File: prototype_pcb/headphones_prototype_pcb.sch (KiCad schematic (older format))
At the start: 51 parts, among them J1 LIGHTING_JACK, J2 CONN_01X10, J3 BOTTOM_FLEX_LIGHTNING, J4 CONN_01X10, J5 LIGHTNING_HEADPHONE_ADAPTER, J6 CONN_01X10, J7 IPHONE_HEADPHONE_JACK, J8 CONN_01X02, U1 SN74LVC1G123, U2 ADG774A, U3 SN74LVC1G123, U4 NC7S32

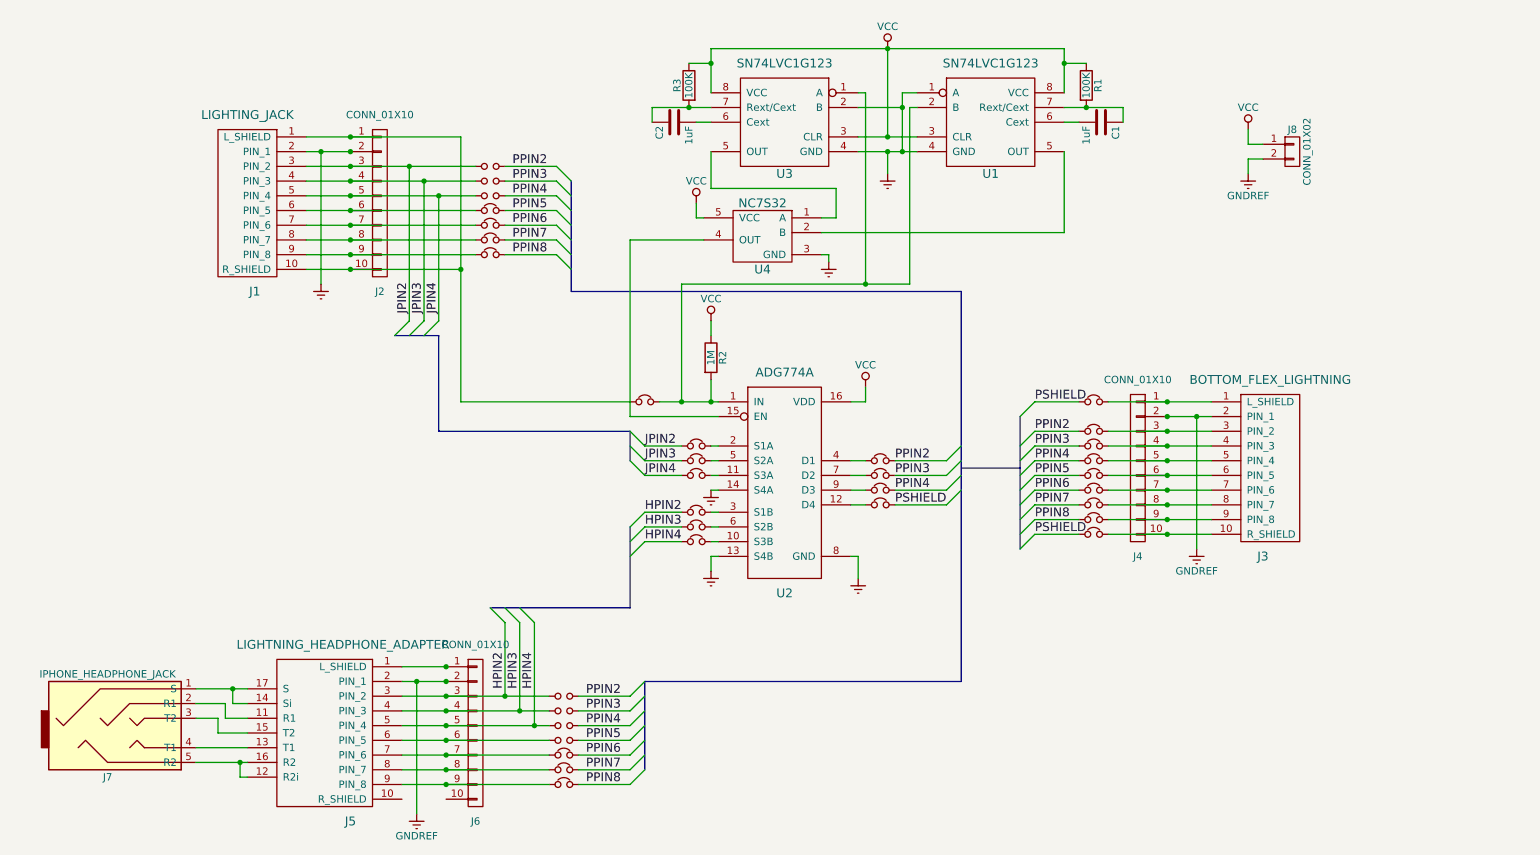
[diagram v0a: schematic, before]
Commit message: Rigid prototype pcb v1.2
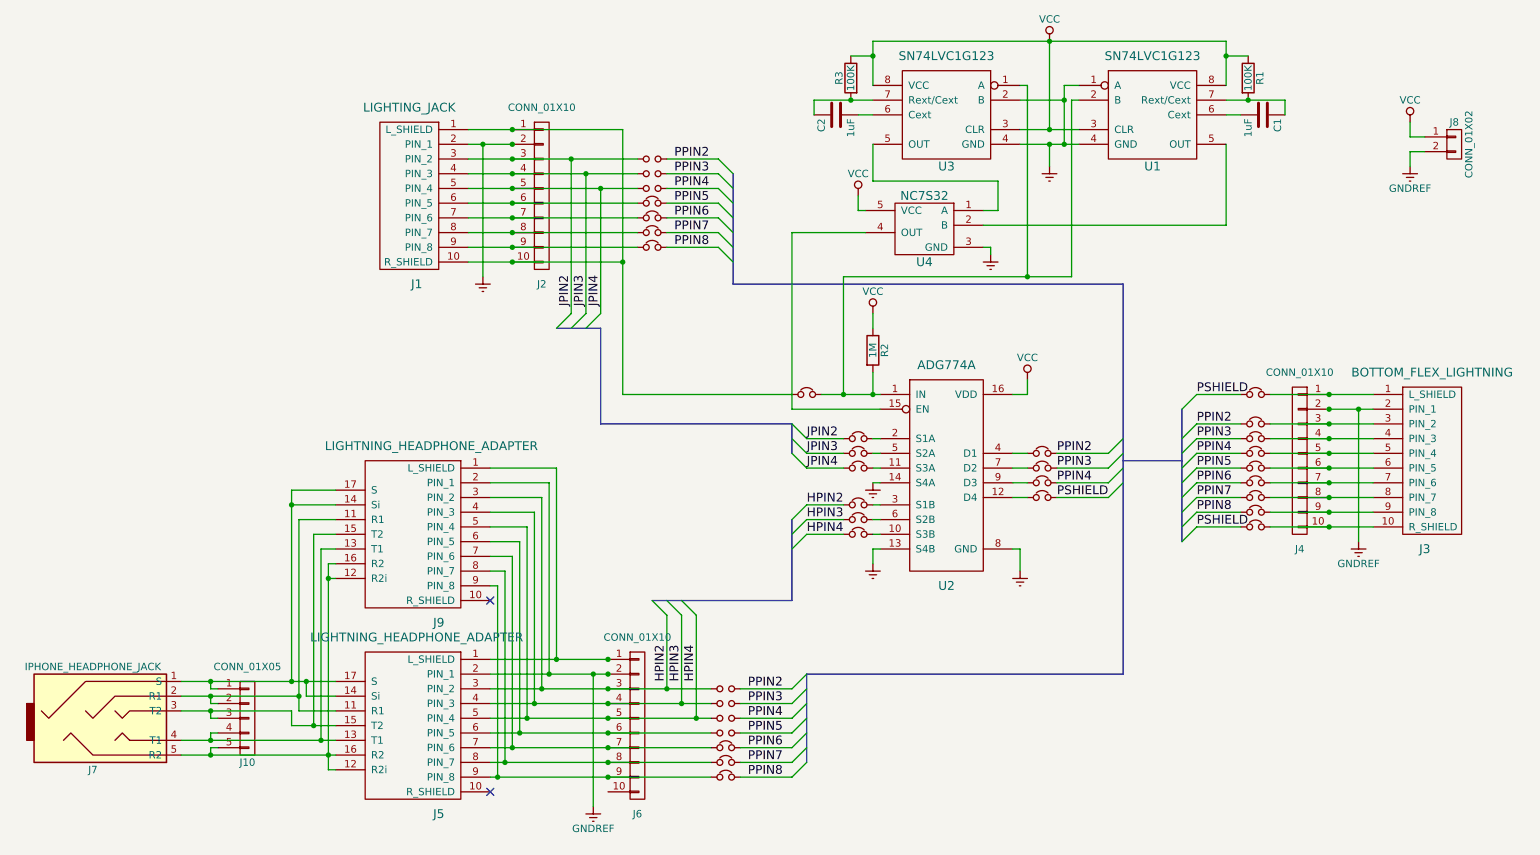
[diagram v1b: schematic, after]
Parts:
- added J10: CONN_01X05, Pin_Headers:Pin_Header_Straight_1x05_Pitch2.54mm, symbol CONN_01X05
- added J9: LIGHTNING_HEADPHONE_ADAPTER, lightning_headphone_adapter:LIGHTNING_HEADPHONE_ADAPTER_HANDWIRE, symbol LIGHTNING_HEADPHONE_ADAPTER
- J5: footprint lightning_headphone_adapter:LIGHTNING_HEADPHONE_ADAPTER -> lightning_headphone_adapter:LIGHTNING_HEADPHONE_ADAPTER_CASTELLATED
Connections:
- net GNDREF: now also J9.2 (PIN_1)
- net HPIN2: now also J9.3 (PIN_2)
- net HPIN3: now also J9.4 (PIN_3)
- net HPIN4: now also J9.5 (PIN_4)
- net at J5.1 (L_SHIELD), J6.1 (P1): now also J9.1 (L_SHIELD)
- net at J5.6 (PIN_5), J6.6 (P6), JP31.1: now also J9.6 (PIN_5)
- net at J5.7 (PIN_6), J6.7 (P7), JP32.1: now also J9.7 (PIN_6)
- net at J5.8 (PIN_7), J6.8 (P8), JP33.1: now also J9.8 (PIN_7)
- net at J5.9 (PIN_8), J6.9 (P9), JP34.1: now also J9.9 (PIN_8)
- net at J5.14 (Si), J5.17 (S), J7.1 (S): now also J10.1 (P1), J9.14 (Si), J9.17 (S)
- net at J5.11 (R1), J7.2 (R1): now also J10.2 (P2), J9.11 (R1)
- net at J5.15 (T2), J7.3 (T2): now also J10.3 (P3), J9.15 (T2)
- net at J5.13 (T1), J7.4 (T1): now also J10.4 (P4), J9.13 (T1)
- net at J5.12 (R2i), J5.16 (R2), J7.5 (R2): now also J10.5 (P5), J9.12 (R2i), J9.16 (R2)
- no-connect marks 0 -> 2
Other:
- moved on the sheet: C1, C2, J1, J2, J3, J4, J5, J6, J7, J8, R1, R2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
